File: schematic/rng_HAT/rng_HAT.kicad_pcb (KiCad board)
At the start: 2 copper layers, 56.5 x 65 mm, 53 parts, among them J1 RPi_GPIO, J2 Conn_01x04_Pin, Q1 2N3904, Q2 2N3904, Q3 2N3904, Q4 BC107, Q5 2N3904, U1 TL072CP, U3 STM32F103C8Tx, Y2 8MHz

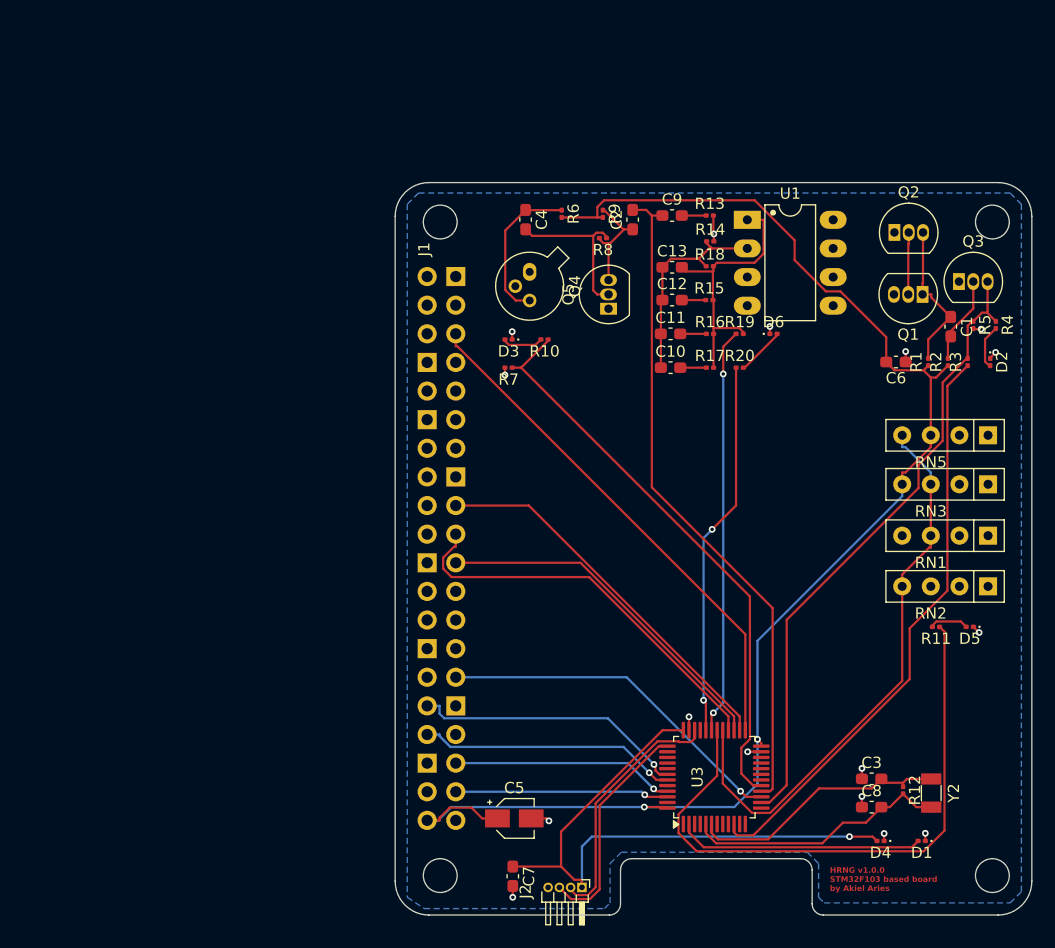
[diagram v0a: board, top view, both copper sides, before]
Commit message: readme
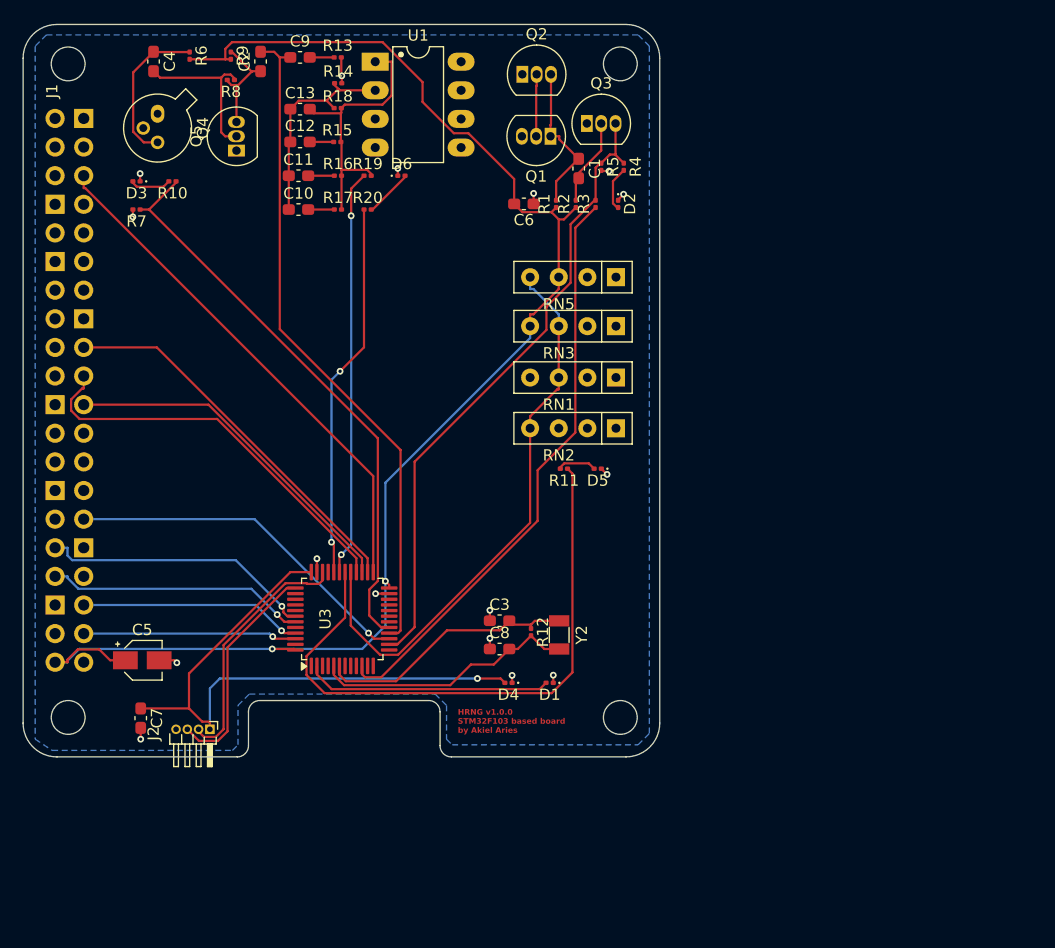
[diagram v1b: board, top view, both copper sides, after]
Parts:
- moved C3 35.9 mm to (167.2, 121.5)
- moved C10 35.9 mm to (149.3, 85.0)
- moved C11 35.9 mm to (149.3, 82.0)
- moved C13 35.9 mm to (149.5, 76.1)
- moved C6 35.9 mm to (169.3, 84.5)
- moved C7 35.9 mm to (135.3, 130.1)
- moved C8 35.9 mm to (167.2, 124.0)
- moved D3 35.9 mm to (135.0, 82.5)
- moved J1 35.9 mm to (128.9, 101.0)
- moved Q3 35.9 mm to (174.9, 77.3)
- moved Q4 35.9 mm to (136.8, 76.5)
- moved Q5 35.9 mm to (143.8, 79.7)
- moved R10 35.9 mm to (138.2, 82.5)
- moved R16 35.9 mm to (152.8, 82.0)
- moved R17 35.9 mm to (152.8, 85.0)
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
